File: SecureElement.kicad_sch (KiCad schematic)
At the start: 3 parts, among them IC7 STSAFA110S8OCD03

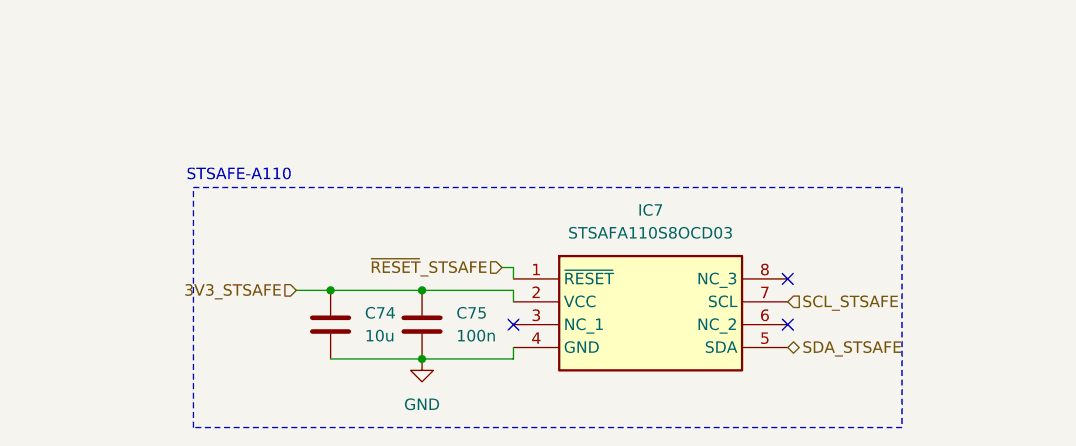
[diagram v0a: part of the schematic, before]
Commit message: Update schematic to Kicad 10
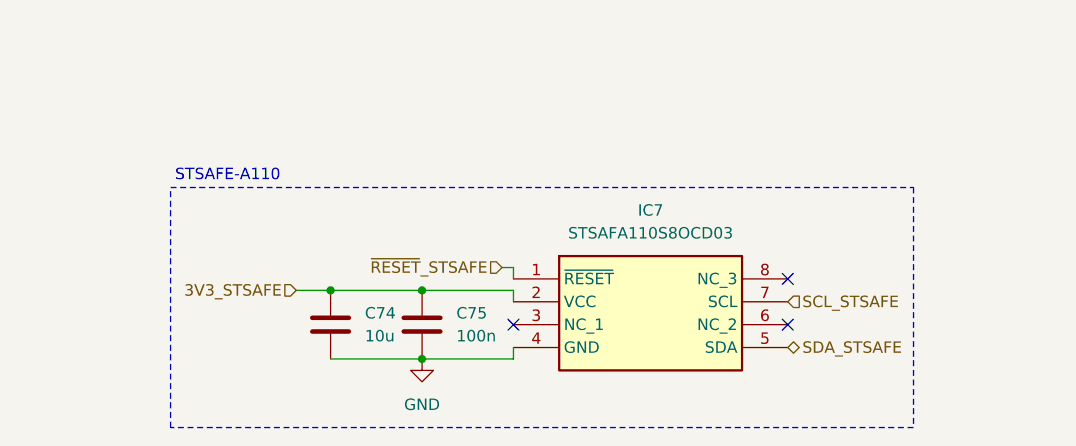
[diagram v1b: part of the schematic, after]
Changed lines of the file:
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@@
 (kicad_sch
-	(version 20250114)
+	(version 20260306)
 	(generator "eeschema")
-	(generator_version "9.0")
+	(generator_version "10.0")
 	(paper "A4")
 	(title_block
@@
 	)
 	(rectangle
-		(start 100.33 80.01)
-		(end 179.07 106.68)
+		(start 97.79 80.01)
+		(end 180.34 106.68)
 		(stroke
 			(width 0)
@@
 	(text "STSAFE-A110"
 		(exclude_from_sim no)
-		(at 105.41 78.74 0)
+		(at 104.14 78.74 0)
 		(effects
 			(font
@@
 		(at 125.73 99.06 0)
 		(unit 1)
+		(body_style 1)
 		(exclude_from_sim no)
 		(in_bom yes)
 		(on_board yes)
+		(in_pos_files yes)
 		(dnp no)
 		(fields_autoplaced yes)
 		(property "Reference" "#PWR0119"
 			(at 125.73 105.41 0)
-			(effects
-				(font
-					(size 1.27 1.27)
-				)
-				(hide yes)
+			(hide yes)
+			(show_name no)
+			(do_not_autoplace no)
+			(effects
+				(font
+					(size 1.27 1.27)
+				)
 			)
 		)
 		(property "Value" "GND"
 			(at 125.73 104.14 0)
+			(show_name no)
+			(do_not_autoplace no)
 			(effects
 				(font
@@
 		(property "Footprint" ""
 			(at 125.73 99.06 0)
-			(effects
-				(font
-					(size 1.27 1.27)
-				)
-				(hide yes)
+			(hide yes)
+			(show_name no)
+			(do_not_autoplace no)
+			(effects
+				(font
+					(size 1.27 1.27)
+				)
 			)
 		)
 		(property "Datasheet" ""
 			(at 125.73 99.06 0)
-			(effects
-				(font
-					(size 1.27 1.27)
-				)
-				(hide yes)
+			(hide yes)
+			(show_name no)
+			(do_not_autoplace no)
+			(effects
+				(font
+					(size 1.27 1.27)
+				)
 			)
 		)
 		(property "Description" "Power symbol creates a global label with name \"GND\" , ground"
 			(at 125.73 99.06 0)
-			(effects
-				(font
-					(size 1.27 1.27)
-				)
-				(hide yes)
+			(hide yes)
+			(show_name no)
+			(do_not_autoplace no)
+			(effects
+				(font
+					(size 1.27 1.27)
+				)
 			)
 		)
@@
 		)
 		(instances
-			(project ""
+			(project "weather-station-poc"
 				(path "/38eb53bb-294e-46e4-ad59-fd355ca373b9/9a031817-cce8-41f5-9861-f61338edb684"
 					(reference "#PWR0119")
@@
 		(at 115.57 95.25 0)
 		(unit 1)
+		(body_style 1)
 		(exclude_from_sim no)
 		(in_bom yes)
 		(on_board yes)
+		(in_pos_files yes)
 		(dnp no)
 		(fields_autoplaced yes)
 		(property "Reference" "C74"
 			(at 119.38 93.9799 0)
+			(show_name no)
+			(do_not_autoplace no)
 			(effects
 				(font
@@
 		(property "Value" "10u"
 			(at 119.38 96.5199 0)
+			(show_name no)
+			(do_not_autoplace no)
 			(effects
 				(font
@@
 		(property "Footprint" "Capacitor_SMD:C_0603_1608Metric_Pad1.08x0.95mm_HandSolder"
 			(at 116.5352 99.06 0)
-			(effects
-				(font
-					(size 1.27 1.27)
-				)
-				(hide yes)
-			)
-		)
-		(property "Datasheet" "~"
+			(hide yes)
+			(show_name no)
+			(do_not_autoplace no)
+			(effects
+				(font
+					(size 1.27 1.27)
+				)
+			)
+		)
+		(property "Datasheet" ""
 			(at 115.57 95.25 0)
-			(effects
-				(font
-					(size 1.27 1.27)
-				)
-				(hide yes)
+			(hide yes)
+			(show_name no)
+			(do_not_autoplace no)
+			(effects
+				(font
+					(size 1.27 1.27)
+				)
 			)
 		)
 		(property "Description" "Unpolarized capacitor"
 			(at 115.57 95.25 0)
-			(effects
-				(font
-					(size 1.27 1.27)
-				)
-				(hide yes)
+			(hide yes)
+			(show_name no)
+			(do_not_autoplace no)
+			(effects
+				(font
+					(size 1.27 1.27)
+				)
 			)
 		)
@@
 		(at 135.89 90.17 0)
 		(unit 1)
+		(body_style 1)
 		(exclude_from_sim no)
 		(in_bom yes)
 		(on_board yes)
+		(in_pos_files yes)
 		(dnp no)
 		(fields_autoplaced yes)
 		(property "Reference" "IC7"
 			(at 151.13 82.55 0)
+			(show_name no)
+			(do_not_autoplace no)
 			(effects
 				(font
@@
 		(property "Value" "STSAFA110S8OCD03"
 			(at 151.13 85.09 0)
+			(show_name no)
+			(do_not_autoplace no)
 			(effects
 				(font
@@
 		(property "Footprint" "weather-station-poc-fp:SOIC127P600X175-8N"
 			(at 162.56 185.09 0)
-			(effects
-				(font
-					(size 1.27 1.27)
-				)
-				(justify left top)
-				(hide yes)
+			(hide yes)
+			(show_name no)
+			(do_not_autoplace no)
+			(effects
+				(font
+					(size 1.27 1.27)
+				)
+				(justify left top)
 			)
 		)
 		(property "Datasheet" "https://www.st.com/resource/en/datasheet/stsafe-a110.pdf"
 			(at 162.56 285.09 0)
-			(effects
-				(font
-					(size 1.27 1.27)
-				)
-				(justify left top)
-				(hide yes)
+			(hide yes)
+			(show_name no)
+			(do_not_autoplace no)
+			(effects
+				(font
+					(size 1.27 1.27)
+				)
+				(justify left top)
 			)
 		)
 		(property "Description" "Authentication, state-of-the-art security for peripherals and IoT devices"
 			(at 135.89 90.17 0)
-			(effects
-				(font
-					(size 1.27 1.27)
-				)
-				(hide yes)
+			(hide yes)
+			(show_name no)
+			(do_not_autoplace no)
+			(effects
+				(font
+					(size 1.27 1.27)
+				)
 			)
 		)
 		(property "Height" "1.75"
 			(at 162.56 485.09 0)
-			(effects
-				(font
-					(size 1.27 1.27)
-				)
-				(justify left top)
-				(hide yes)
+			(hide yes)
+			(show_name no)
+			(do_not_autoplace no)
+			(effects
+				(font
+					(size 1.27 1.27)
+				)
+				(justify left top)
 			)
 		)
 		(property "Mouser Part Number" "511-STSAFA110S8OCD03"
 			(at 162.56 585.09 0)
-			(effects
-				(font
-					(size 1.27 1.27)
-				)
-				(justify left top)
-				(hide yes)
+			(hide yes)
+			(show_name no)
+			(do_not_autoplace no)
+			(effects
+				(font
+					(size 1.27 1.27)
+				)
+				(justify left top)
 			)
 		)
 		(property "Mouser Price/Stock" "https://www.mouser.co.uk/ProductDetail/STMicroelectronics/STSAFA110S8OCD03?qs=7%2F6SraaimPRtuR%252B2wUZjKw%3D%3D"
 			(at 162.56 685.09 0)
-			(effects
-				(font
-					(size 1.27 1.27)
-				)
-				(justify left top)
-				(hide yes)
+			(hide yes)
+			(show_name no)
+			(do_not_autoplace no)
+			(effects
+				(font
+					(size 1.27 1.27)
+				)
+				(justify left top)
 			)
 		)
 		(property "Manufacturer_Name" "STMicroelectronics"
 			(at 162.56 785.09 0)
-			(effects
-				(font
-					(size 1.27 1.27)
-				)
-				(justify left top)
-				(hide yes)
+			(hide yes)
+			(show_name no)
+			(do_not_autoplace no)
+			(effects
+				(font
+					(size 1.27 1.27)
+				)
+				(justify left top)
 			)
 		)
 		(property "Manufacturer_Part_Number" "STSAFA110S8OCD03"
 			(at 162.56 885.09 0)
-			(effects
-				(font
-					(size 1.27 1.27)
-				)
-				(justify left top)
-				(hide yes)
+			(hide yes)
+			(show_name no)
+			(do_not_autoplace no)
+			(effects
+				(font
+					(size 1.27 1.27)
+				)
+				(justify left top)
 			)
 		)
@@
 		)
 		(instances
-			(project ""
+			(project "weather-station-poc"
 				(path "/38eb53bb-294e-46e4-ad59-fd355ca373b9/9a031817-cce8-41f5-9861-f61338edb684"
 					(reference "IC7")
@@
 		(at 125.73 95.25 0)
 		(unit 1)
+		(body_style 1)
 		(exclude_from_sim no)
 		(in_bom yes)
 		(on_board yes)
+		(in_pos_files yes)
 		(dnp no)
 		(fields_autoplaced yes)
 		(property "Reference" "C75"
 			(at 129.54 93.9799 0)
+			(show_name no)
+			(do_not_autoplace no)
 			(effects
 				(font
@@
 		(property "Value" "100n"
 			(at 129.54 96.5199 0)
+			(show_name no)
+			(do_not_autoplace no)
 			(effects
 				(font
@@
 		(property "Footprint" "Capacitor_SMD:C_0603_1608Metric_Pad1.08x0.95mm_HandSolder"
 			(at 126.6952 99.06 0)
-			(effects
-				(font
-					(size 1.27 1.27)
-				)
-				(hide yes)
-			)
-		)
-		(property "Datasheet" "~"
+			(hide yes)
+			(show_name no)
+			(do_not_autoplace no)
+			(effects
+				(font
+					(size 1.27 1.27)
+				)
+			)
+		)
+		(property "Datasheet" ""
 			(at 125.73 95.25 0)
-			(effects
-				(font
-					(size 1.27 1.27)
-				)
-				(hide yes)
+			(hide yes)
+			(show_name no)
+			(do_not_autoplace no)
+			(effects
+				(font
+					(size 1.27 1.27)
+				)
 			)
 		)
 		(property "Description" "Unpolarized capacitor"
 			(at 125.73 95.25 0)
-			(effects
-				(font
-					(size 1.27 1.27)
-				)
-				(hide yes)
-			)
-		)
+			(hide yes)
+			(show_name no)
+			(do_not_autoplace no)
+			(effects
+				(font
+					(size 1.27 1.27)
+				)
+			)
+		)
